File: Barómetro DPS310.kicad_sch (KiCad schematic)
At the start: 4 parts, among them U5 DPS310XTSA1

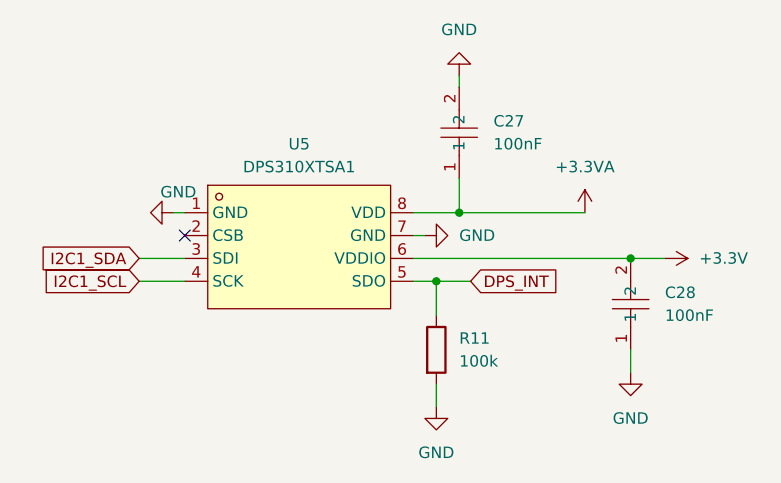
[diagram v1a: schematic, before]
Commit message: Avance 02/08
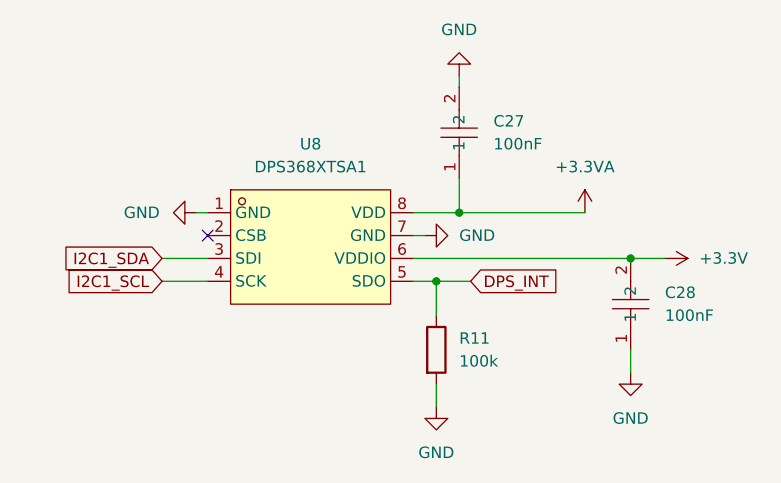
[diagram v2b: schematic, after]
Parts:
- removed U5: DPS310XTSA1, ARLISS-footprints:LGA-8_DPS310XTSA1, symbol CANSAT_STM32_symbols:DPS310XTSA1
- added U8: DPS368XTSA1, easyeda2kicad:LGA-8_L2.5-W2.0-P0.65-TR_DPS368, symbol CANSAT_STM32_symbols:DPS368XTSA1
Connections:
- net +3.3V: now also U8.6 (VDDIO)
- net +3.3VA: now also U8.8 (VDD)
- net DPS_INT: now also U8.5 (SDO)
- net GND: now also U8.1 (GND), U8.7 (GND)
- net I2C1_SCL: now also U8.4 (SCK)
- net I2C1_SDA: now also U8.3 (SDI)
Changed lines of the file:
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@@
 	)
 	(no_connect
-		(at 153.67 92.71)
+		(at 156.21 92.71)
 	)
 	(wire
 		(pts
-			(xy 148.59 97.79) (xy 153.67 97.79)
+			(xy 151.13 97.79) (xy 156.21 97.79)
 		)
 		(stroke
@@
 	(wire
 		(pts
-			(xy 152.4 90.17) (xy 153.67 90.17)
+			(xy 154.94 90.17) (xy 156.21 90.17)
 		)
 		(stroke
@@
 	(wire
 		(pts
-			(xy 148.59 95.25) (xy 153.67 95.25)
+			(xy 151.13 95.25) (xy 156.21 95.25)
 		)
 		(stroke
@@
 	(global_label "I2C1_SDA"
 		(shape input)
-		(at 148.59 95.25 180)
+		(at 151.13 95.25 180)
 		(fields_autoplaced yes)
 		(effects
@@
 		)
 		(property "Intersheetrefs" "${INTERSHEET_REFS}"
-			(at 136.7753 95.25 0)
+			(at 139.3153 95.25 0)
 			(hide yes)
 			(show_name no)
@@
 	(global_label "I2C1_SCL"
 		(shape input)
-		(at 148.59 97.79 180)
+		(at 151.13 97.79 180)
 		(fields_autoplaced yes)
 		(effects
@@
 		)
 		(property "Intersheetrefs" "${INTERSHEET_REFS}"
-			(at 136.8358 97.79 0)
+			(at 139.3758 97.79 0)
 			(hide yes)
 			(show_name no)
@@
 	(symbol
 		(lib_id "power:GND")
-		(at 152.4 90.17 270)
+		(at 154.94 90.17 270)
 		(unit 1)
 		(body_style 1)
@@
 		(dnp no)
 		(property "Reference" "#PWR063"
-			(at 146.05 90.17 0)
+			(at 148.59 90.17 0)
 			(hide yes)
 			(show_name no)
@@
 		)
 		(property "Value" "GND"
-			(at 154.94 87.884 90)
+			(at 150.876 90.17 90)
 			(show_name no)
 			(do_not_autoplace no)
@@
 		)
 		(property "Footprint" ""
-			(at 152.4 90.17 0)
+			(at 154.94 90.17 0)
 			(hide yes)
 			(show_name no)
@@
 		)
 		(property "Datasheet" ""
-			(at 152.4 90.17 0)
+			(at 154.94 90.17 0)
 			(hide yes)
 			(show_name no)
@@
 		)
 		(property "Description" "Power symbol creates a global label with name \"GND\" , ground"
-			(at 152.4 90.17 0)
+			(at 154.94 90.17 0)
 			(hide yes)
 			(show_name no)
@@
 	)
 	(symbol
-		(lib_id "CANSAT_STM32_symbols:DPS310XTSA1")
-		(at 166.37 93.98 0)
+		(lib_id "CANSAT_STM32_symbols:DPS368XTSA1")
+		(at 167.64 93.98 0)
 		(unit 1)
 		(body_style 1)
@@
 		(dnp no)
 		(fields_autoplaced yes)
-		(property "Reference" "U5"
-			(at 166.37 82.55 0)
+		(property "Reference" "U8"
+			(at 167.64 82.55 0)
 			(show_name no)
 			(do_not_autoplace no)
@@
 			)
 		)
-		(property "Value" "DPS310XTSA1"
-			(at 166.37 85.09 0)
+		(property "Value" "DPS368XTSA1"
+			(at 167.64 85.09 0)
 			(show_name no)
 			(do_not_autoplace no)
@@
 			)
 		)
-		(property "Footprint" "ARLISS-footprints:LGA-8_DPS310XTSA1"
-			(at 166.37 105.41 0)
+		(property "Footprint" "easyeda2kicad:LGA-8_L2.5-W2.0-P0.65-TR_DPS368"
+			(at 167.64 105.41 0)
 			(hide yes)
 			(show_name no)
@@
 			)
 		)
-		(property "Datasheet" "https://lcsc.com/product-detail/Sensors_Infineon_DPS310XTSA1_DPS310XTSA1_C130156.html"
-			(at 166.37 107.95 0)
+		(property "Datasheet" "https://www.lcsc.com/datasheet/C3232508.pdf"
+			(at 167.64 107.95 0)
 			(hide yes)
 			(show_name no)
@@
 		)
 		(property "Description" ""
-			(at 166.37 93.98 0)
+			(at 167.64 93.98 0)
 			(hide yes)
 			(show_name no)
@@
 			)
 		)
-		(property "MPN" "DPS310"
-			(at 166.37 113.03 0)
+		(property "Manufacturer" "Infineon(英飞凌)"
+			(at 167.64 110.49 0)
 			(hide yes)
 			(show_name no)
@@
 			)
 		)
-		(property "LCSC Part" "C130156"
-			(at 166.37 115.57 0)
+		(property "MPN" "DPS368XTSA1"
+			(at 167.64 113.03 0)
 			(hide yes)
 			(show_name no)
@@
 			)
 		)
-		(property "Field7" ""
-			(at 166.37 93.98 0)
+		(property "LCSC Part" "C3232508"
+			(at 167.64 115.57 0)
 			(hide yes)
 			(show_name no)
@@
 			)
 		)
-		(pin "5"
+		(pin "2"
 		)
 		(pin "1"
 		)
-		(pin "6"
-		)
-		(pin "8"
-		)
 		(pin "4"
 		)
-		(pin "7"
+		(pin "5"
 		)
 		(pin "3"
 		)
-		(pin "2"
+		(pin "6"
+		)
+		(pin "8"
+		)
+		(pin "7"
 		)
 		(instances
 			(project "ARLISS_STM32_2026"
 				(path "/9719ea46-14c4-4409-9c57-49dd5454c03f/9e299f07-4887-409a-8623-587b30453872"
-					(reference "U5")
+					(reference "U8")
 					(unit 1)
 				)
